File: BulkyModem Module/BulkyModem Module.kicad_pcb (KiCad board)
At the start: 2 copper layers, 100 x 100 mm, 81 parts, among them J1 DC IN, J2 DCE, J3 Module_Panel, J5 C64_Modem_OUT, K1 HK19F-DC, M1 Mounting, M2 Mounting, M3 Mounting, M4 Mounting, SW1 SET_1200, U1 74HCT244, U2 74HCT04, U3 MAX232, U4 MAX232, U5 74HCT04, U6 74HCT32

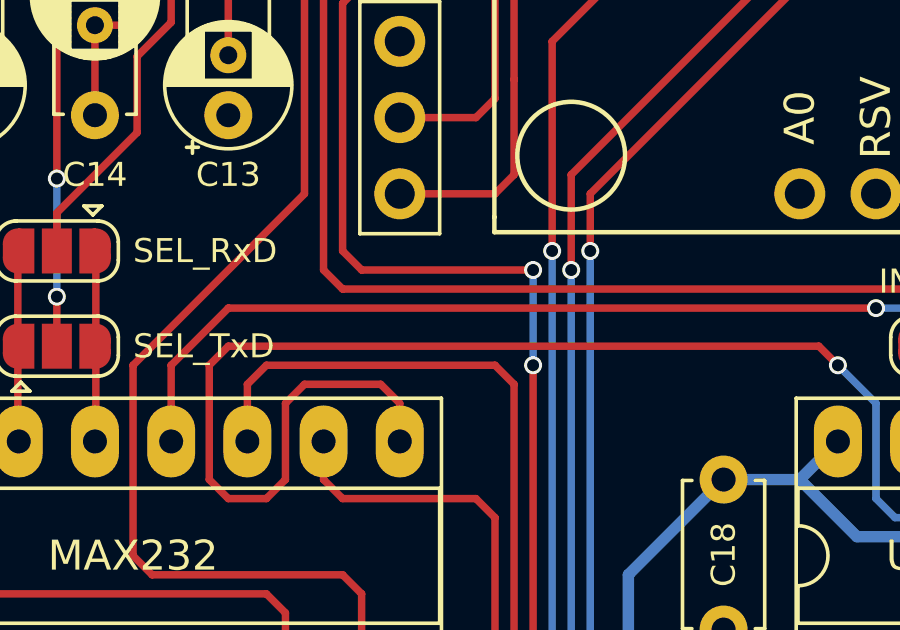
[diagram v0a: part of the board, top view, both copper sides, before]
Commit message: Just clarification
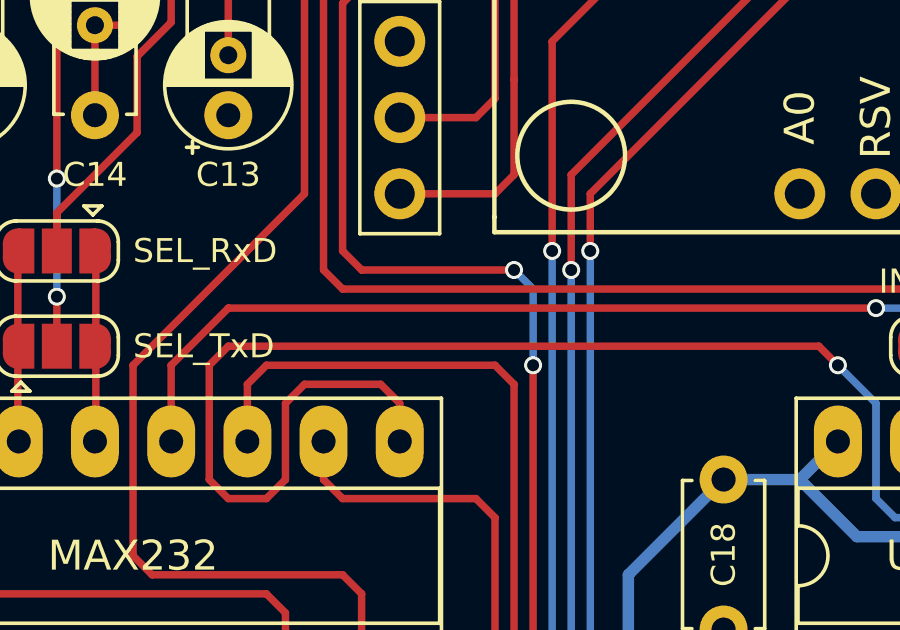
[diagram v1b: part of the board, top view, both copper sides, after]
